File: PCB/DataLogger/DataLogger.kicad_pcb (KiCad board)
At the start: 2 copper layers, 59.5 x 46 mm, 35 parts, among them J1 Power, J10 Screw_Terminal_01x02, J2 1WI Screw_Terminal_01x03, J3 1WI Screw_Terminal_01x03, J4 1WI Screw_Terminal_01x03, J5 I²C_Screw_Terminal_01x04, J6 I²C_Screw_Terminal_01x04, J7 Screw_Terminal_01x04, J8 Screw_Terminal_01x02, J9 Screw_Terminal_01x02

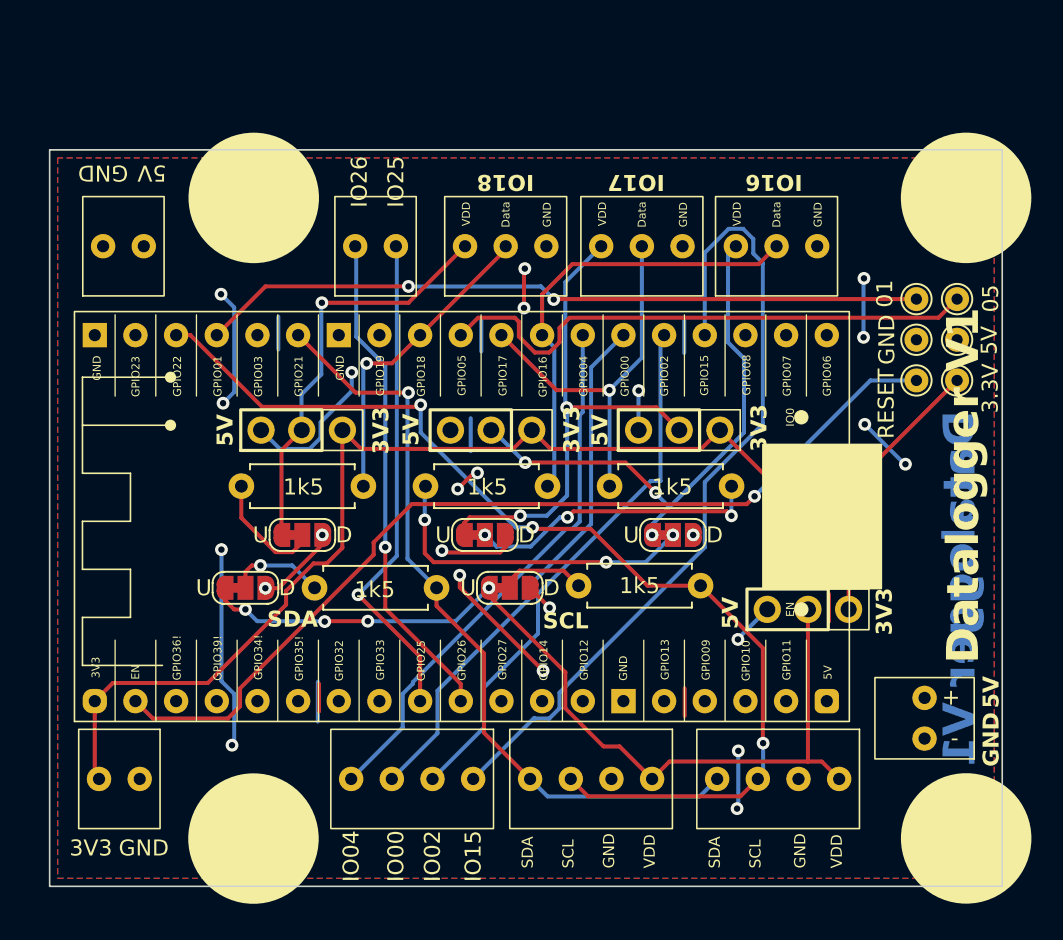
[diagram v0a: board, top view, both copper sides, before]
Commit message: PCB V1.2
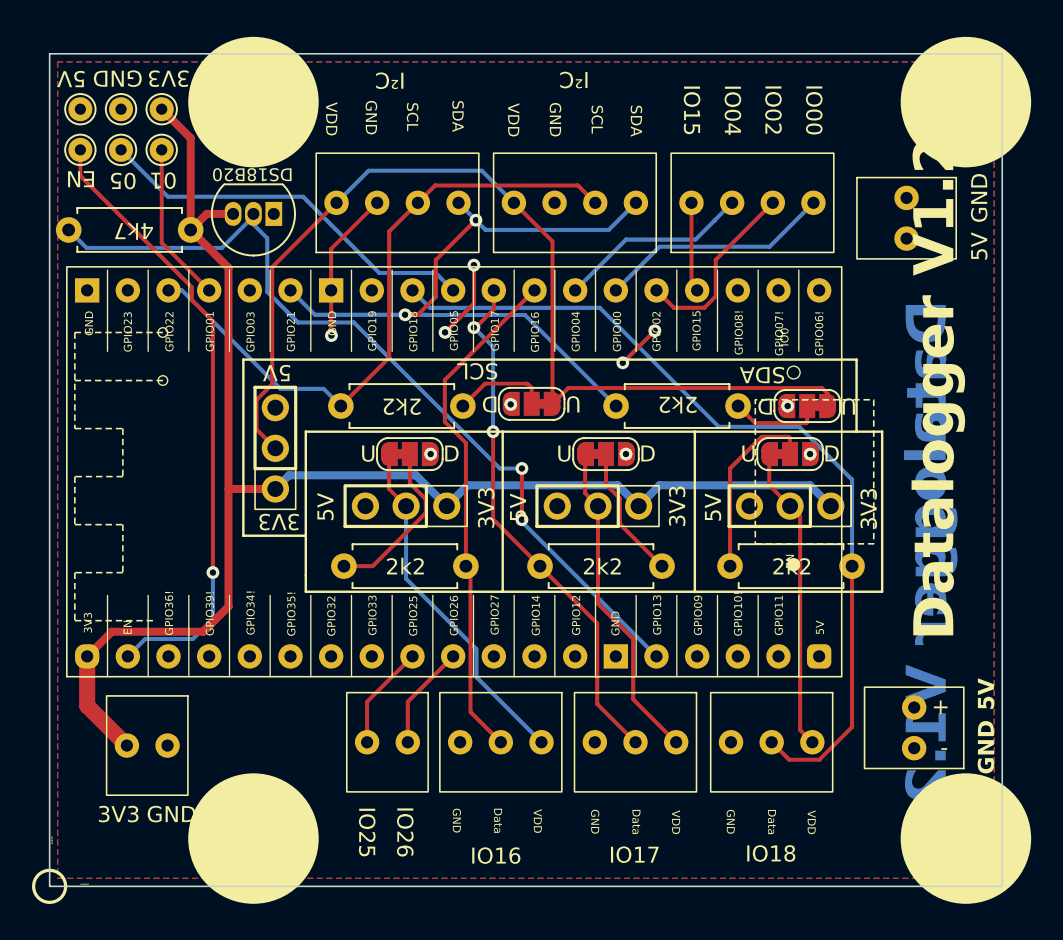
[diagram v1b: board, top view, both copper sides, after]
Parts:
- removed J1: Power, ESP32Board:Screw Terminal 2*2.54 Power
- removed J4: 1WI Screw_Terminal_01x03, ESP32Board:Screw Terminal 3*2.54 1WI
- removed J5, J6: I²C_Screw_Terminal_01x04, ESP32Board:Screw Terminal 4*2.54 I²C
- removed the REF** at (118.0, 111.8)
- removed the REF** at (118.0, 151.8)
- removed the REF** at (162.5, 151.8)
- removed the REF** at (162.5, 111.8)
- added 1WI3: 1WI Screw_Terminal_01x03, ESP32Board:Screw Terminal 3*2.54 1WI, F.Cu at (146.5, 145.8)
- added I²C1: I²C_Screw_Terminal_01x04, ESP32Board:Screw Terminal 4*2.54 I²C, F.Cu at (143.1, 112.1)
- added I²C2: I²C_Screw_Terminal_01x04, ESP32Board:Screw Terminal 4*2.54 I²C, F.Cu at (132.1, 112.1)
- added Power1: Power, ESP32Board:Screw Terminal 2*2.54 Power, F.Cu at (159.2, 142.3)
- added R4: 4k7, Resistor_THT:R_Axial_DIN0207_L6.3mm_D2.5mm_P7.62mm_Horizontal, F.Cu at (106.4, 113.8)
- added REF**: MountingHole_4.3mm_M4_ISO14580, MountingHole:MountingHole_4.3mm_M4_ISO14580, F.Cu at (162.5, 105.8)
- added REF**: MountingHole_4.3mm_M4_ISO14580, MountingHole:MountingHole_4.3mm_M4_ISO14580, F.Cu at (162.5, 151.8)
- added REF**: MountingHole_4.3mm_M4_ISO14580, MountingHole:MountingHole_4.3mm_M4_ISO14580, F.Cu at (118.0, 151.8)
- added REF**: MountingHole_4.3mm_M4_ISO14580, MountingHole:MountingHole_4.3mm_M4_ISO14580, F.Cu at (118.0, 105.8)
- added U2: DS18B20, Package_TO_SOT_THT:TO-92_Inline, F.Cu at (119.2, 112.8)
- ExtraGPIO2: renamed from J10; value Screw_Terminal_01x02 -> Screw_Terminal_01x
- R1, R10, R2, R3, R9: value 1k5 -> 2k2
- TP3: value 3.3V -> 3V3
- TP4: value RESET -> EN
- moved TP1 56.6 mm to (107.2, 106.2), turned to 0 degrees
- moved TP4 54.2 mm to (107.2, 108.8), turned to 0 degrees
- moved TP6 53.0 mm to (109.7, 108.8), turned to 180 degrees
- moved TP3 52.5 mm to (112.2, 106.2), turned to 0 degrees
- moved TP2 51.7 mm to (109.7, 106.2), turned to 0 degrees
- moved TP5 48.1 mm to (112.2, 108.8), turned to 180 degrees
- moved ExtraGPIO1 47.8 mm to (154.2, 112.1), turned to 90 degrees
- moved J8 46.4 mm to (158.8, 115.6), turned to 0 degrees
- moved 1WI2 39.7 mm to (129.6, 145.8), turned to -90 degrees
- moved JP9 36.9 mm to (152.6, 124.8), turned to 180 degrees
- moved JP4 33.2 mm to (119.3, 124.9), turned to 0 degrees
- moved 1WI1 32.0 mm to (138.0, 145.8), turned to -90 degrees
- moved ExtraGPIO2 31.3 mm to (123.8, 145.8), turned to -90 degrees
- moved R3 30.9 mm to (147.7, 134.8)
- moved JP7 30.9 mm to (151.5, 127.8)
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- renumbered J2 to 1WI1, J3 to 1WI2, J7 to ExtraGPIO1
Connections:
- net Net-(J10-Pin_1) renamed /IO25
- net Net-(J10-Pin_2) renamed /IO26
- net Net-(J2-Data) renamed /IO17
- net Net-(J3-Data) renamed /IO16
- net Net-(J4-Data) renamed /IO18
- net Net-(J7-Pin_4) renamed /IO15
- net Net-(U1-1) renamed /IO01
- net Net-(U1-5) renamed /IO05
- net Net-(U1-RESET) renamed /RESET
- ExtraGPIO1 pad 1: Net-(J7-Pin_1) -> /IO00
- ExtraGPIO1 pad 2: Net-(J7-Pin_2) -> /IO02
- ExtraGPIO1 pad 3: Net-(J7-Pin_3) -> /IO04
- U1 pad 15: unconnected-(U1-13-Pad15) -> /IO13
- U1 pad 24: Net-(J7-Pin_3) -> /IO02
- U1 pad 25: Net-(J7-Pin_2) -> /IO00
- U1 pad 26: Net-(J7-Pin_1) -> /IO04
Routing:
- net +5V: track 55.5 -> 0.00 mm, vias 16 -> 0
- net /IO13: track 0.00 -> 53.9 mm, vias 0 -> 2
- net /IO15: track 51.1 -> 5.62 mm
- net /IO01: track 45.3 -> 10.0 mm, vias 2 -> 0
- net /IO18: track 19.6 -> 54.3 mm, vias 1 -> 0
- net Net-(J7-Pin_3): track 34.1 -> 0.00 mm
- net Net-(J7-Pin_1): track 33.9 -> 0.00 mm
- net Net-(J7-Pin_2): track 33.7 -> 0.00 mm
- net Net-(I²C1-SCL): track 66.8 -> 40.4 mm, vias 3 -> 0
- net /IO26: track 31.1 -> 6.54 mm, vias 1 -> 0
- net /IO25: track 31.0 -> 6.54 mm, vias 1 -> 0
- net /RESET: track 59.1 -> 39.0 mm
- net GND: track 34.9 -> 17.3 mm, vias 11 -> 10
- net /IO00: track 0.00 -> 14.6 mm
- net Net-(1WI2-VDD): track 34.2 -> 21.9 mm, vias 3 -> 0
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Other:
- board size 59.5 x 46 mm -> 59.5 x 52 mm
- board text added: "Datalogger V1.2"
- board text added: "I²C"
- board text added: "locked"
- board text removed: "Datalogger V1"
